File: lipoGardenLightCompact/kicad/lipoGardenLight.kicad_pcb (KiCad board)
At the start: 2 copper layers, 65.3 x 33.5 mm, 14 parts, among them Q1 BC557, Q2 SS8050, Q3 SS8050

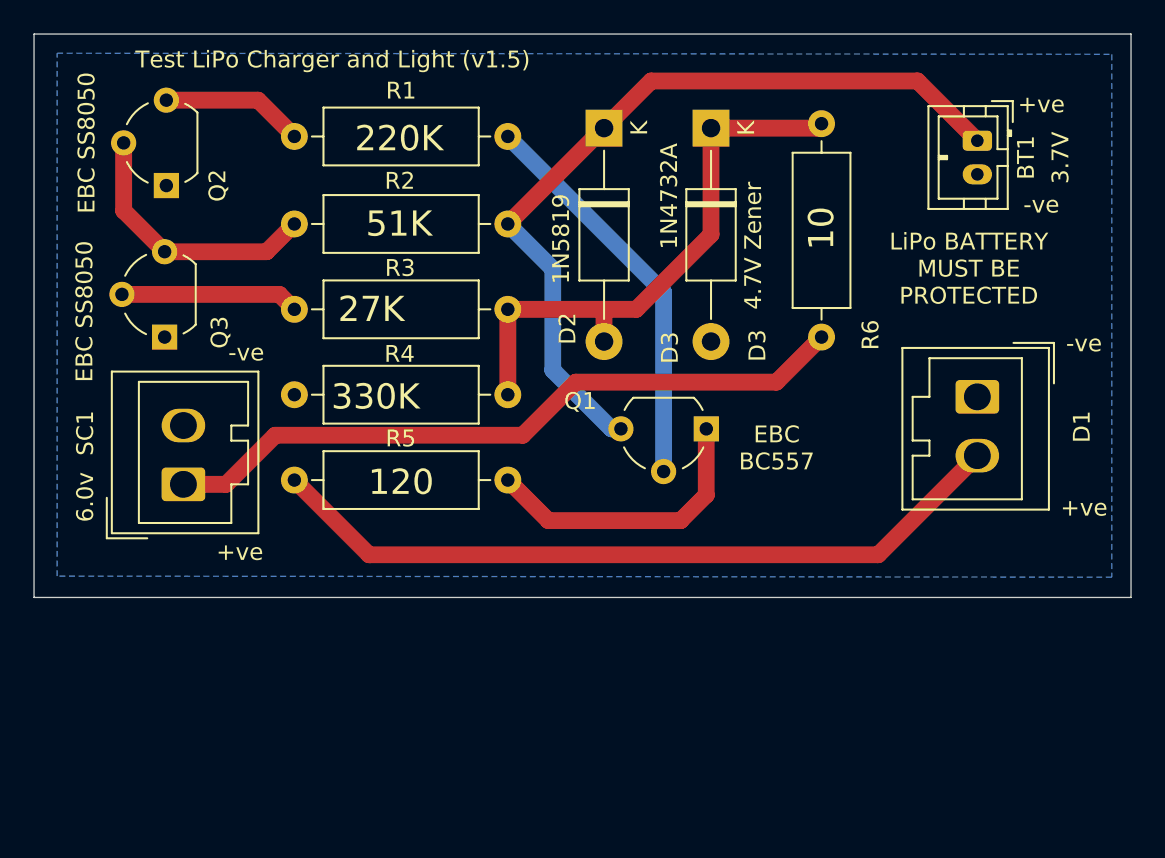
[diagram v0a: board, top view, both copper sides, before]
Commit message: Kicad 8 / minor tweaks
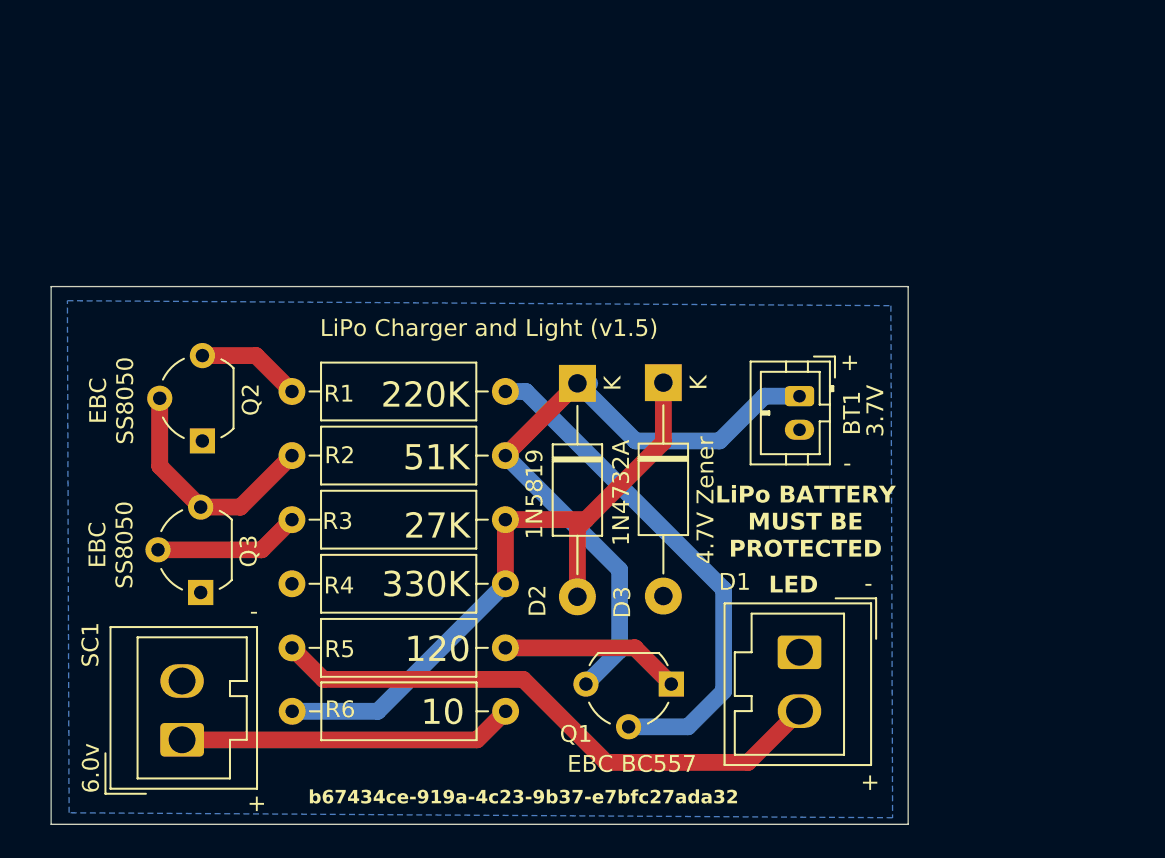
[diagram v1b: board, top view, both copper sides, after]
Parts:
- moved R6 47.1 mm to (125.3, 70.3), turned to 0 degrees
- moved D1 18.5 mm to (155.5, 66.8)
- moved BT1 18.5 mm to (155.5, 51.5)
- moved D3 15.4 mm to (147.4, 50.7)
- moved Q2 15.3 mm to (120.0, 54.2)
- moved Q3 15.3 mm to (119.9, 63.2)
- moved Q1 15.3 mm to (147.9, 68.7)
- moved D2 15.3 mm to (142.3, 50.8)
- moved SC1 15.2 mm to (118.8, 72.0)
- moved R1 15.2 mm to (125.3, 51.2)
- moved R2 13.8 mm to (125.3, 55.1)
- moved R3 12.5 mm to (125.3, 58.9)
- moved R4 11.3 mm to (125.3, 62.7)
- moved R5 9.98 mm to (125.3, 66.5)
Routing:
- net Net-(SC1-+): track 41.6 -> 20.0 mm
- net Net-(D1-A): track 44.9 -> 34.3 mm
- net Net-(BT1-+): track 48.2 -> 39.8 mm
- net Net-(Q1-B): track 23.8 -> 30.5 mm
- net Net-(Q1-C): track 17.4 -> 10.8 mm
- net Net-(D2-A): track 34.0 -> 39.3 mm
- net Net-(Q2-C): track 8.51 -> 6.21 mm
- net Net-(Q3-B): track 10.6 -> 8.71 mm
- net Net-(Q2-B): track 15.9 -> 14.2 mm
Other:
- board size 65.3 x 33.5 mm -> 51 x 32 mm
- board text added: "+"
- board text added: "-"
- board text added: "3.7V LiPo - Must have protection circuit. 6.0V Solar Panel"
- board text added: "LED"
- board text added: "LiPo Charger and Light (v1.5)"
- board text added: "b67434ce-919a-4c23-9b37-e7bfc27ada32"
- board text removed: "+ve"
- board text removed: "-ve"
- board text removed: "D3"
- board text removed: "Test LiPo Charger and Light (v1.5)"
- board text removed: "Test PCB for debugging 3.7V LiPo - Must have protection circuit. 6.0V Solar Panel"
